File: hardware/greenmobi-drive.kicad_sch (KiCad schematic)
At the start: 17 parts, among them J1 USB_C_Receptacle_USB2.0_14P, J3 BAT, J4 CAN, J5 Sensors, U2 TJA1051T-3

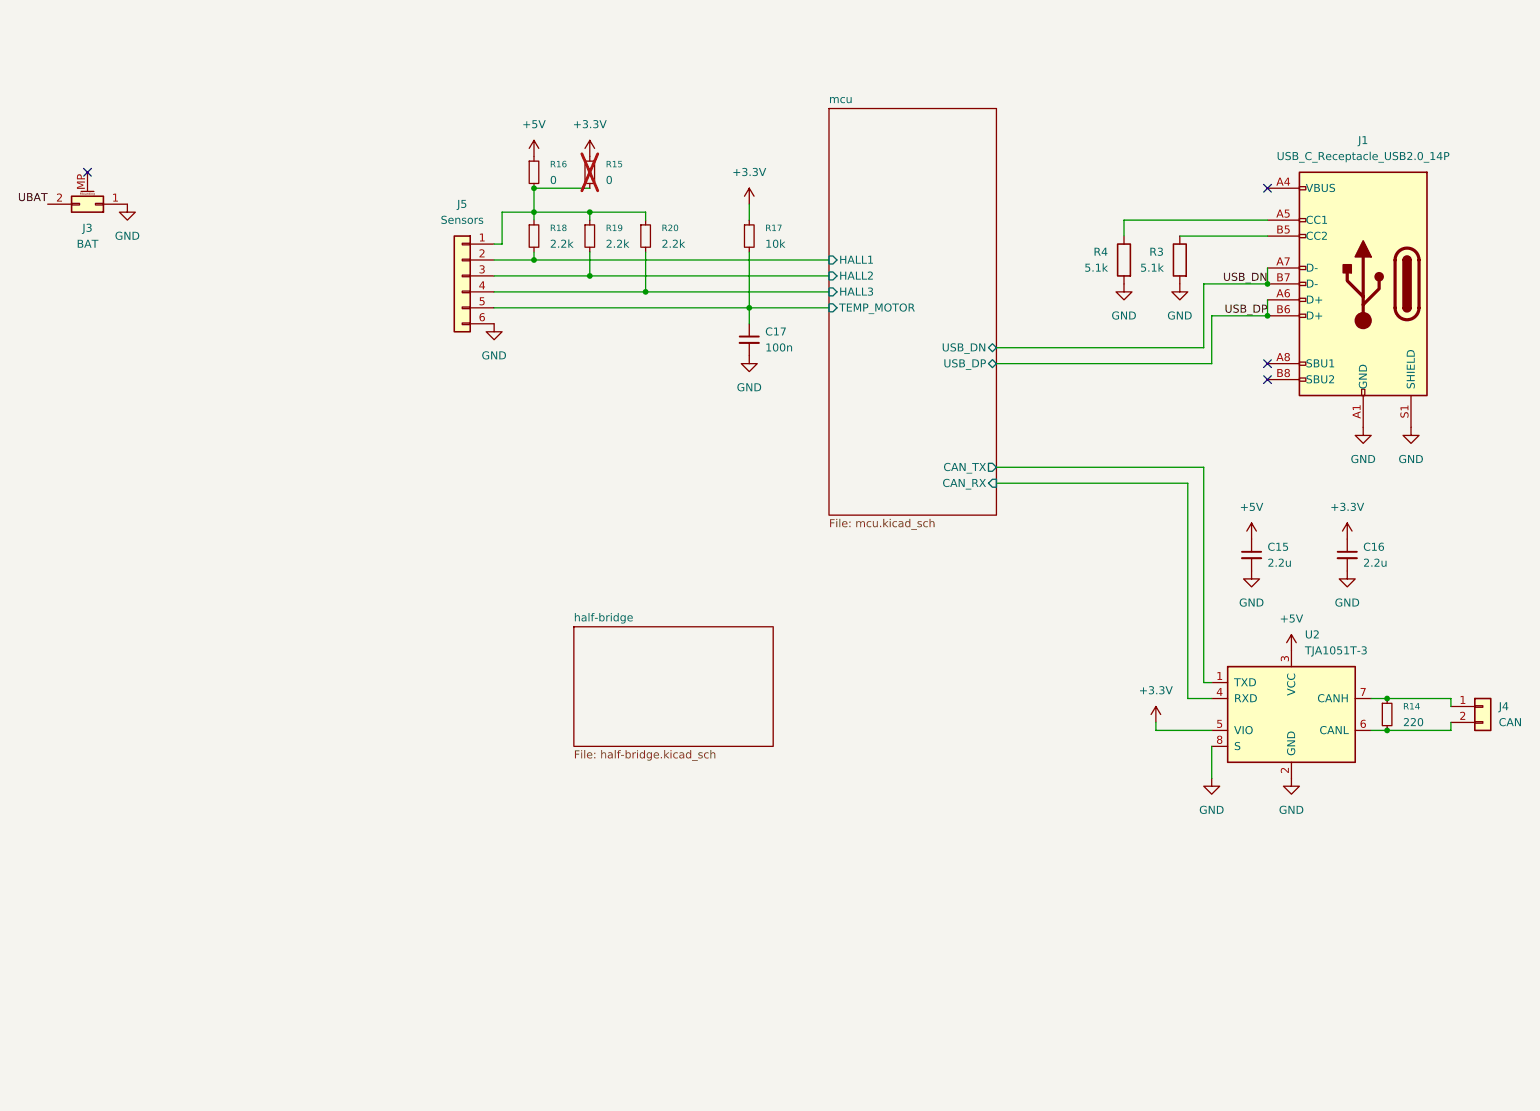
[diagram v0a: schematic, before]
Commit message: half bridges
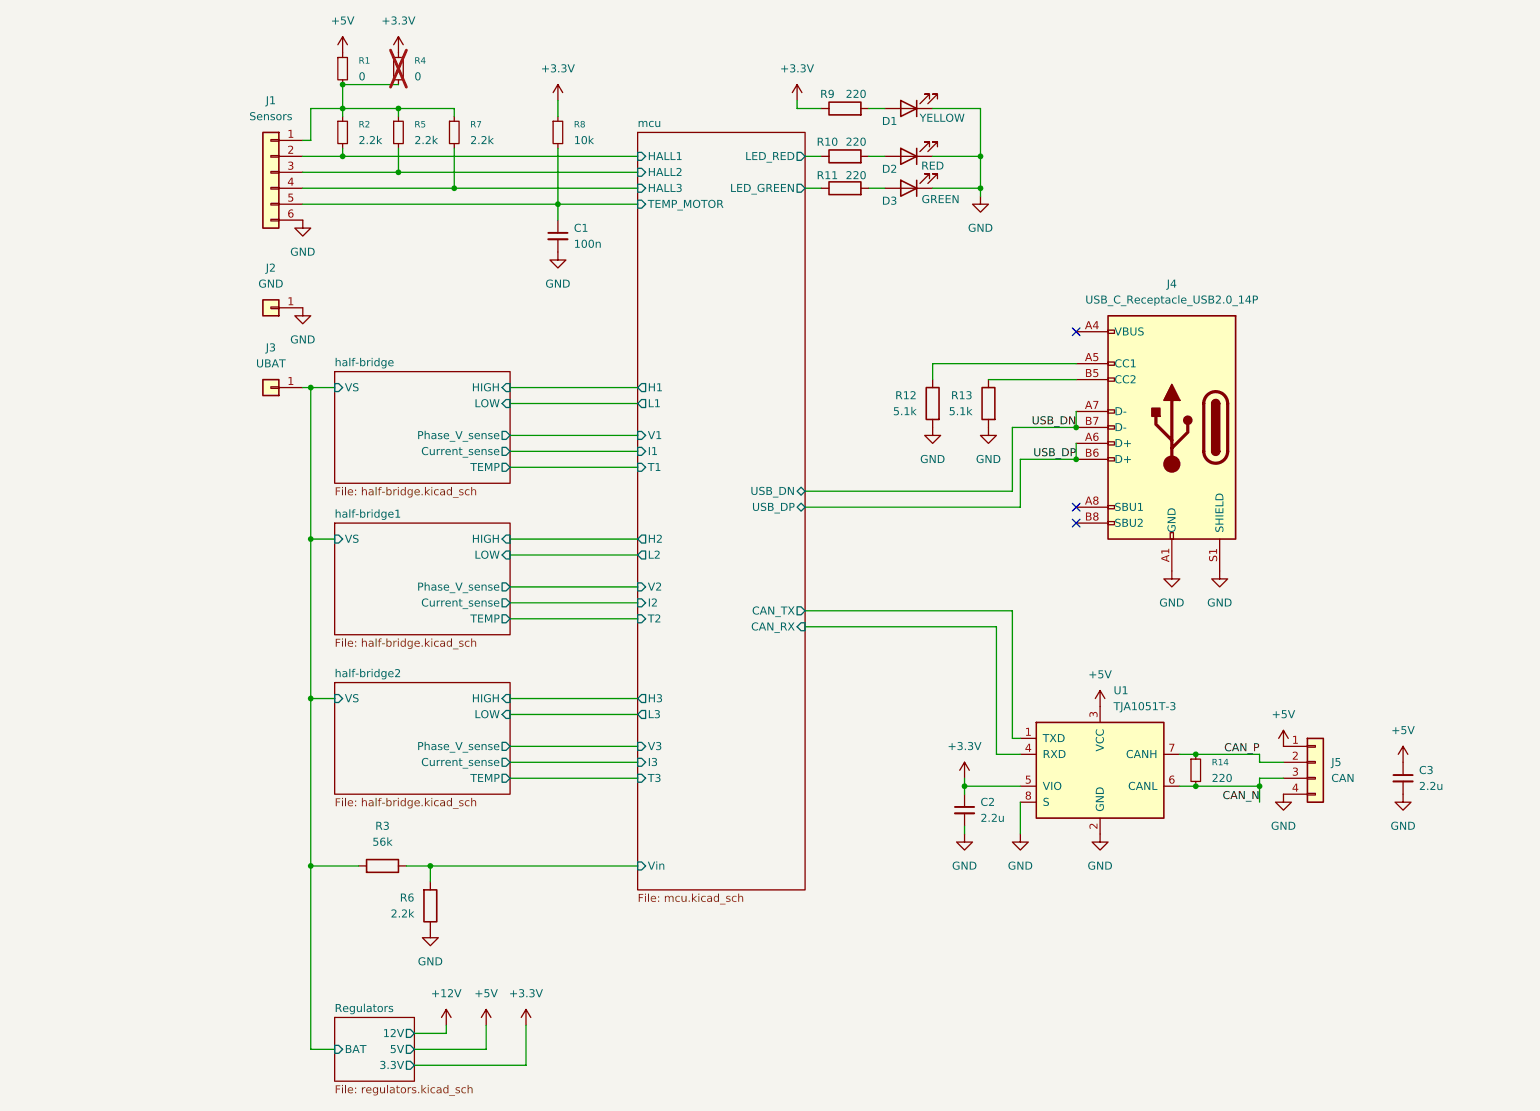
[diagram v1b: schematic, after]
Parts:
- removed J3: BAT, Connector_AMASS:AMASS_XT90PW-M_1x02_P10.90mm_Horizontal, symbol Connector_Generic_MountingPin:Conn_02x01_MountingPin
- removed J4: CAN, symbol Connector_Generic:Conn_01x02
- added D1: YELLOW, LED_SMD:LED_0805_2012Metric, symbol Device:LED
- added D2: RED, LED_SMD:LED_0805_2012Metric, symbol Device:LED
- added D3: GREEN, LED_SMD:LED_0805_2012Metric, symbol Device:LED
- added J2: GND, MountingHole:MountingHole_5.3mm_M5_DIN965_Pad, symbol Connector_Generic:Conn_01x01
- added J3: UBAT, MountingHole:MountingHole_5.3mm_M5_DIN965_Pad, symbol Connector_Generic:Conn_01x01
- added J5: CAN, Connector_JST:JST_GH_SM04B-GHS-TB_1x04-1MP_P1.25mm_Horizontal, symbol Connector_Generic:Conn_01x04
- added R10, R11, R9: 220, symbol Device:R
- added R3: 56k, Resistor_SMD:R_0402_1005Metric, symbol Device:R
- added R6: 2.2k, symbol Device:R
- C2: renamed from C16; footprint (none) -> Capacitor_SMD:C_0402_1005Metric
- C3: renamed from C15; footprint (none) -> Capacitor_SMD:C_0402_1005Metric
- renumbered C17 to C1, J5 to J1, J1 to J4, R16 to R1, R4 to R12, R3 to R13, R18 to R2, R15 to R4, R19 to R5, R20 to R7, R17 to R8, U2 to U1
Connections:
- net +3.3V: now also R9.1
- net +5V: now also J5.1 (Pin_1)
- net GND: now also D1.1 (K), D2.1 (K), D3.1 (K), J2.1 (Pin_1), J5.4 (Pin_4), R6.1
- net CAN_P: now reaches R14.1, U1.7 (CANH)
- net CAN_P: now also J5.2 (Pin_2)
- net CAN_N: now reaches R14.2, U1.6 (CANL)
- net CAN_N: now also J5.3 (Pin_3)
- new net: D2.2 (A), R10.2
- new net: D1.2 (A), R9.2
- new net: D3.2 (A), R11.2
- new net Regulators/BAT: J3.1 (Pin_1), R3.2
- new net mcu/LED_GREEN: R11.1
- new net mcu/LED_RED: R10.1
- new net mcu/Vin: R3.1, R6.2
- no-connect marks 4 -> 3
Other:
- added sheet Regulators (regulators.kicad_sch)
- added sheet half-bridge1 (half-bridge.kicad_sch)
- added sheet half-bridge2 (half-bridge.kicad_sch)
- sheet half-bridge ports: added Current_sense, HIGH, LOW, Phase_V_sense, TEMP, VS; removed none
- sheet mcu ports: added H1, H2, H3, I1, I2, I3, L1, L2, L3, LED_GREEN, LED_RED, T1, T2, T3, V1, V2, V3, Vin; removed none
- moved on the sheet: C1, C2, C3, J1, J4, R1, R12, R13, R14, R2, R4, R5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
